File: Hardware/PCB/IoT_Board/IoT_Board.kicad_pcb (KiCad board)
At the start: 2 copper layers, 100 x 50 mm, 109 parts, among them IC1 VS1838B, IC2 TPS563200DDCR, J9 USB_C_Receptacle_USB2.0_16P, K1 Relay_SPDT, K2 Relay_SPDT, Q1 AO3400A, Q2 AO3400A, Q3 AO3400A, U1 ESP32-S3-WROOM-1, U2 ME6211C50M5, U5 PC817, U6 PC817

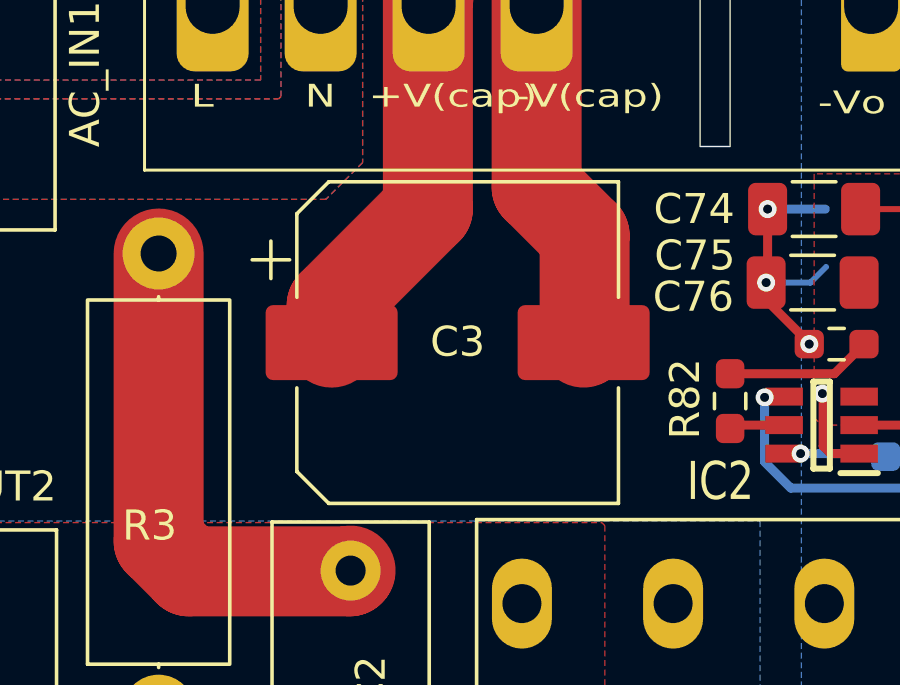
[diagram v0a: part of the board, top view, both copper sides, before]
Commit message: fix nhieu bug
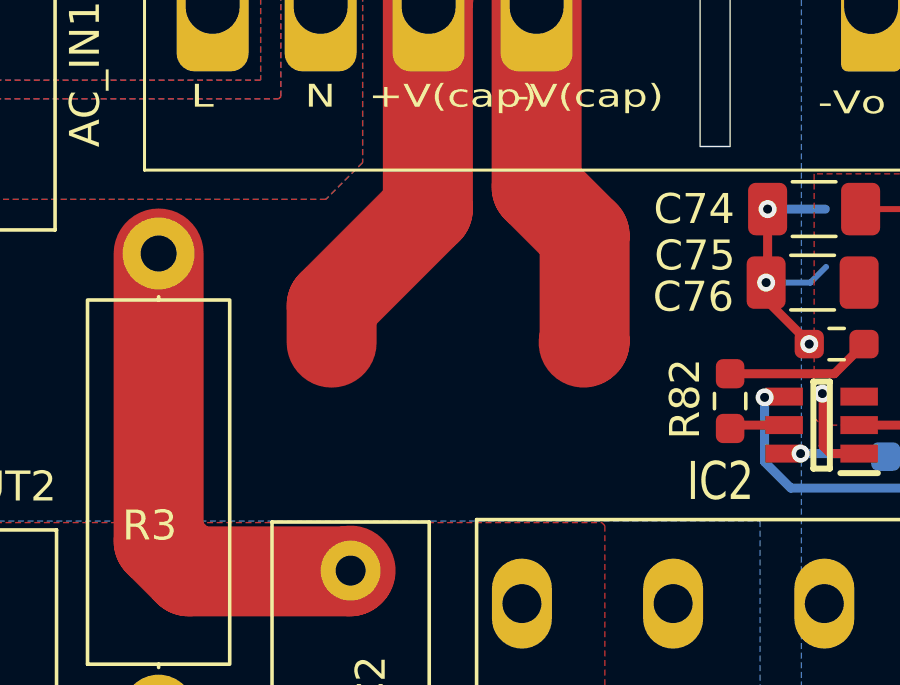
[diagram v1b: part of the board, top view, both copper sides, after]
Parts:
- removed C3: 10uF, Capacitor_SMD:CP_Elec_10x10.5
